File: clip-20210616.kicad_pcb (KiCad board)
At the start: 2 copper layers, 42.9 x 52.1 mm, 38 parts, among them Q1 2.5A/30V, U1 MCP73831, U2 AP2112K-3.3, U3 ESP32-WROOM-32

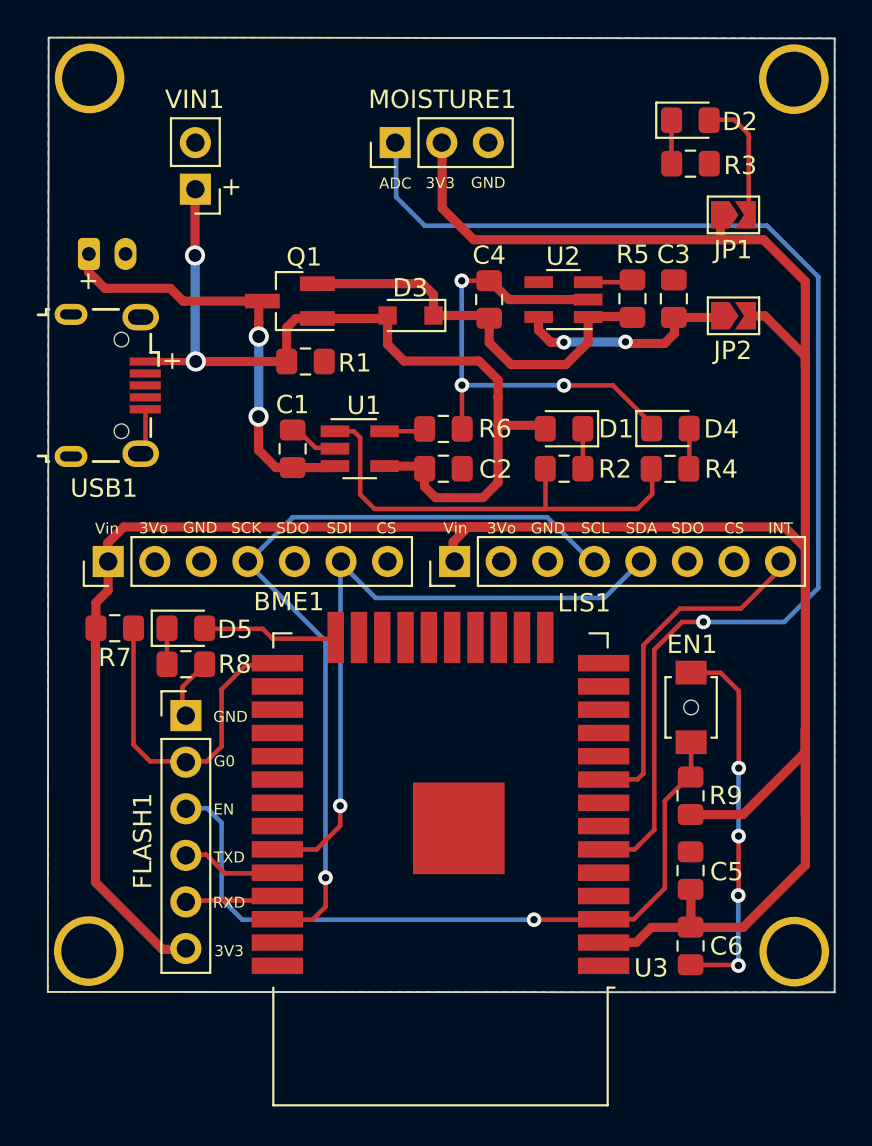
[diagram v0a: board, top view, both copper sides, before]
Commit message: Update design
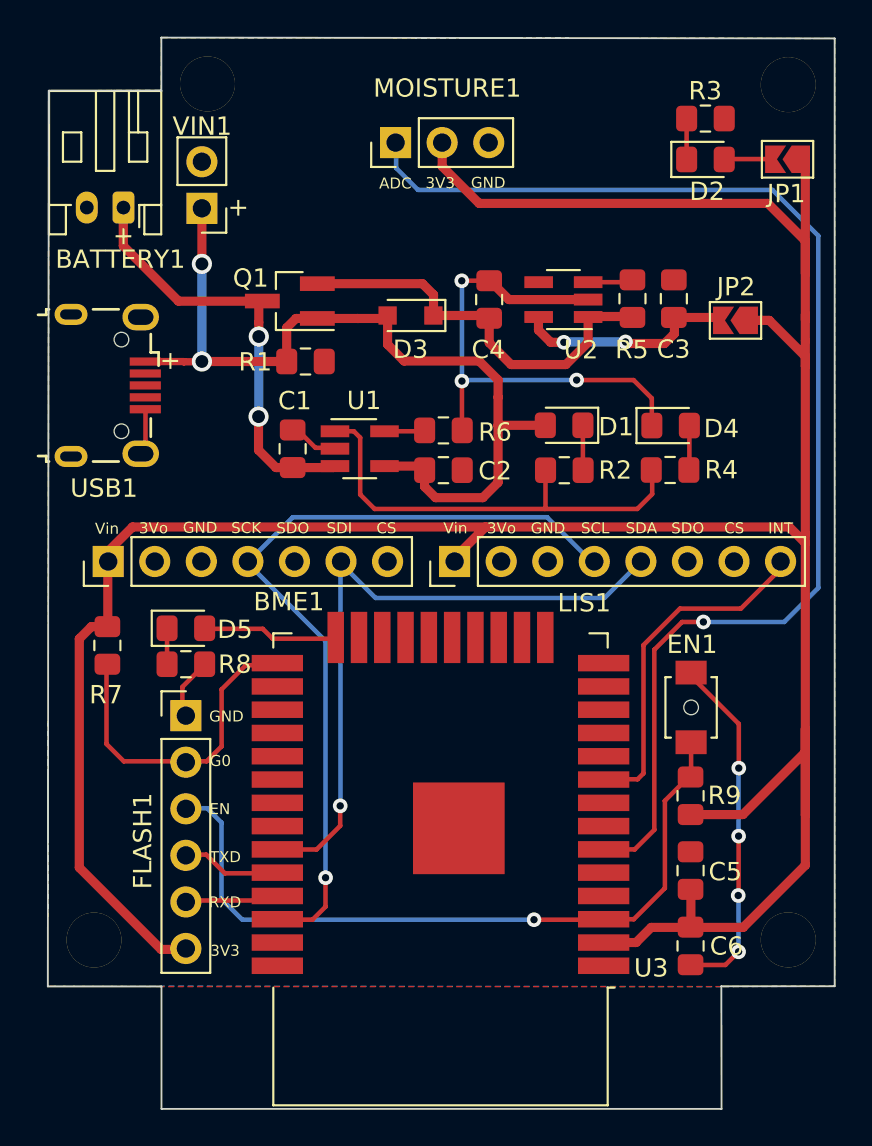
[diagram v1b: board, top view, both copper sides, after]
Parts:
- removed H1, H2, H3, H4: MountingHole, MountingHole:MountingHole_2.2mm_M2_DIN965_Pad
- added REF**: MountingHole_2.2mm_M2_Pad, MountingHole:MountingHole_2.2mm_M2_Pad, F.Cu at (136.1, 75.8)
- added REF**: MountingHole_2.2mm_M2_Pad, MountingHole:MountingHole_2.2mm_M2_Pad, F.Cu at (167.8, 75.8)
- added REF**: MountingHole_2.2mm_M2_Pad, MountingHole:MountingHole_2.2mm_M2_Pad, F.Cu at (129.9, 122.5)
- added REF**: MountingHole_2.2mm_M2_Pad, MountingHole:MountingHole_2.2mm_M2_Pad, F.Cu at (167.8, 122.4)
- BATTERY1: moved to F.Cu
- moved JP1 4.23 mm to (167.8, 79.9), turned to 180 degrees
- moved BATTERY1 3.16 mm to (131.5, 82.5), turned to 180 degrees
- moved R3 2.59 mm to (163.3, 77.6)
- moved D2 2.29 mm to (163.3, 79.9)
- moved VIN1 1.10 mm to (135.8, 82.5)
- moved R7 1.02 mm to (130.7, 106.4), turned to 90 degrees
- moved JP2 0.27 mm to (164.9, 88.6), turned to 180 degrees
- moved D1 0.19 mm to (155.6, 94.4)
- moved D4 0.16 mm to (161.4, 94.4)
- moved R2 0.08 mm to (155.6, 96.8)
- moved R6 0.08 mm to (149.0, 94.7)
- moved C2 0.08 mm to (149.0, 96.8)
- moved R4 0.06 mm to (161.4, 96.8)
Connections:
- JP2 pad 1: Net-(C3-Pad1) -> +3V3
- JP2 pad 2: +3V3 -> Net-(C3-Pad1)
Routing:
- net +3V3: track 160.3 -> 166.3 mm
- net Net-(D2-Pad2): track 7.43 -> 2.54 mm
- net VBUS: track 47.9 -> 46.7 mm
- net GND: track 56.8 -> 56.1 mm
- net Net-(D2-Pad1): track 2.78 -> 2.25 mm
- net +BATT: track 24.8 -> 24.3 mm
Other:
- board size 42.9 x 52.1 mm -> 42.9 x 58.4 mm
